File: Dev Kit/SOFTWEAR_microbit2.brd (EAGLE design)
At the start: 61.1 x 28 mm, 16 parts, among them J1 EDGE-80PTH-RA, J2 M22PTH, J3 QWIIC_RIGHT_ANGLE, X1 SM03B-SRSS-TB, X2 SM03B-SRSS-TB, X3 SM03B-SRSS-TB

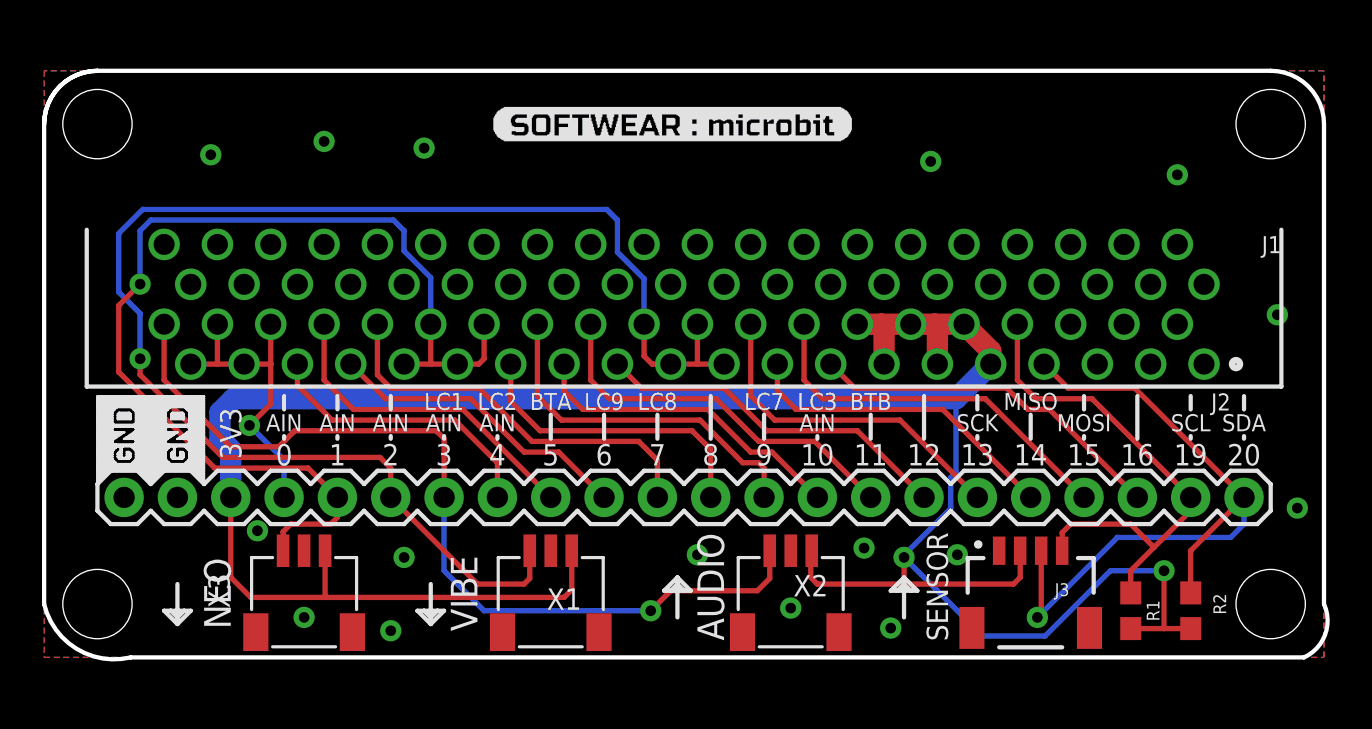
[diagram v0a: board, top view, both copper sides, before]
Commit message: updated design
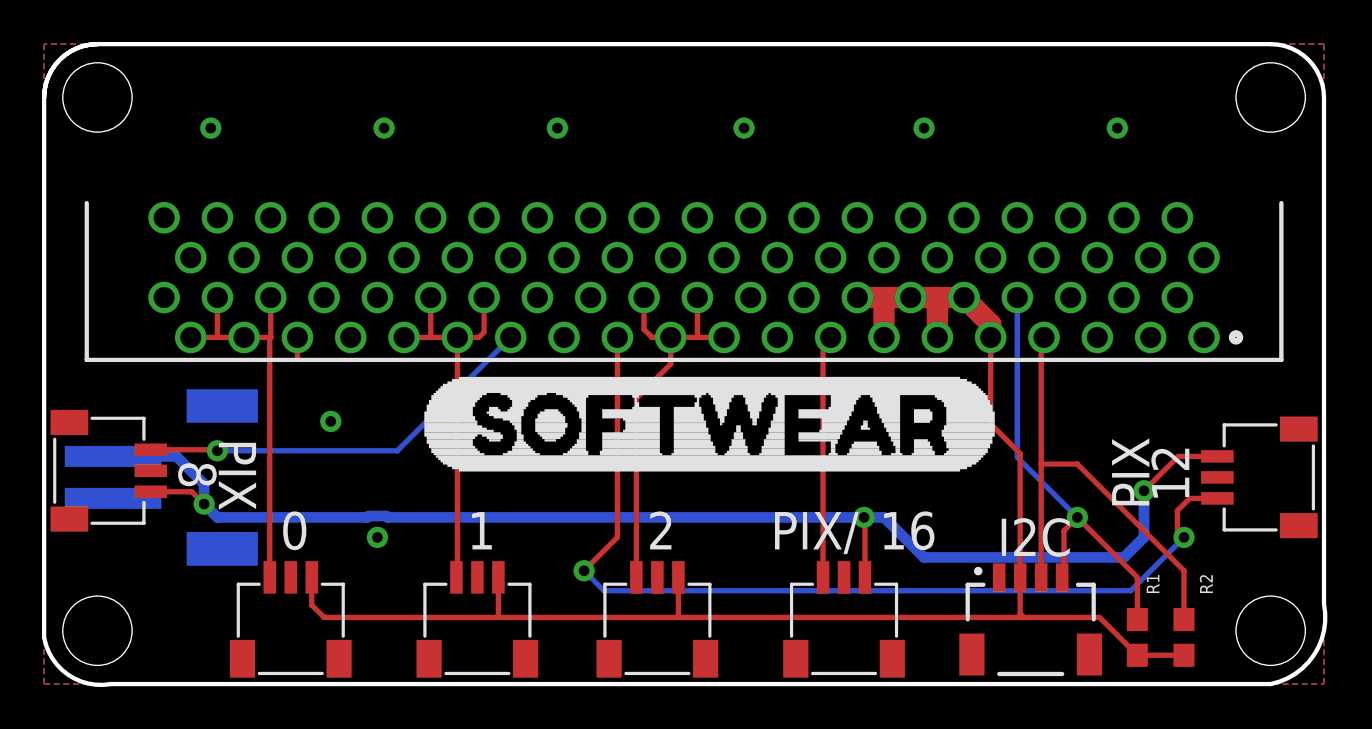
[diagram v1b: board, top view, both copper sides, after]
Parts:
- removed U$2: (no value), negasilk:NEGASILK_MICRO_BIT_BREAKOUT
- removed U$3: (no value), buzzard_labels (21):SOFTWEAR_#_MICROBIT5
- added X4, X5, X6: SM03B-SRSS-TB, con-JST SH (1):SM03B-SRSS-TB
- J2: value M22PTH -> (none); device local_lib:1X22 -> SparkFun-Connectors:JST-2-SMD
- U$1: device negasilk:NEGASILK_MICRO_BIT_BREAKOUT -> buzzard_labels (24):SOFTWEAR0
- moved X2 23.8 mm to (15.6, 5.08)
- moved X3 16.9 mm to (33.0, 5.08)
- moved U$1 15.5 mm to (21.6, 12.4)
- moved X1 3.72 mm to (24.4, 5.08)
- moved J2 3.31 mm to (10.8, 9.84), flipped to the bottom, turned to 90 degrees
- moved R1 1.31 mm to (55.9, 2.22)
- moved R2 1.31 mm to (58.1, 2.22)
- moved J1 1.27 mm to (34.3, 16.5)
- moved H3 1.27 mm to (62.2, 2.54)
- moved H4 1.27 mm to (6.35, 2.54)
- moved H1 1.27 mm to (6.35, 27.9)
- moved H2 1.27 mm to (62.2, 27.9)
- moved J3 1.27 mm to (50.8, 5.08)
- moved FRAME2 0.64 mm to (3.81, -1.27)
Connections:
- removed net 12: J1.A23, J2.16
- removed net 16: J1.A15, J2.20
- removed net 8: J1.A27, J2.12
- removed net AUD: J1.A40, J2.7, X2.1
- removed net NEO: J1.A28, J1.A29, J1.A30, J1.A31, J2.5, X3.1
- removed net VIBE: J1.A19, J1.A20, J1.A21, J1.A22, J2.6, X1.1
- new net 1: J1.A28, J1.A29, J1.A30, J1.A31, X1.1
- new net 2: J1.A19, J1.A20, J1.A21, J1.A22, X3.1
- new net 3: J1.A40
- new net NEO1: J1.A27, X4.1
- new net NEO2: J1.A23, X5.1
- new net NEO3: J1.A15, X6.1
- new net V_BATT: J2.2, X4.3, X5.3, X6.3
- net 0: now also X2.1; no longer J2.4
- net 10: no longer J2.14
- net 11: no longer J2.15
- net 13: no longer J2.17
- net 14: no longer J2.18
- net 15: no longer J2.19
- net 3.3V: no longer J2.3
- net 4: no longer J2.8
- net 5: no longer J2.9
- net 6: no longer J2.10
- net 7: no longer J2.11
- net 9: no longer J2.13
- net GND: now also X4.2, X5.2, X6.2; no longer J2.2
- net SCL: no longer J2.21
- net SDA: no longer J2.22
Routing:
- net VIBE: track 69.4 -> 0.00 mm, vias 1 -> 0
- net V_BATT: track 0.00 -> 64.2 mm, vias 0 -> 3
- net NEO: track 50.2 -> 0.00 mm, vias 1 -> 0
- net 3.3V: track 121.5 -> 73.2 mm, vias 2 -> 0
- net NEO2: track 0.00 -> 45.3 mm, vias 0 -> 2
- net AUD: track 42.3 -> 0.00 mm, vias 1 -> 0
- net 2: track 0.00 -> 19.5 mm
- net NEO1: track 0.00 -> 19.4 mm, vias 0 -> 1
- net 7: track 19.2 -> 0.00 mm
- net 1: track 0.00 -> 18.9 mm
- net 15: track 18.3 -> 0.00 mm
- net 11: track 18.3 -> 0.00 mm
- net 12: track 17.2 -> 0.00 mm
- net 16: track 17.2 -> 0.00 mm
- net 9: track 17.0 -> 0.00 mm
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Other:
- board size 61.1 x 28 mm -> 61 x 30.5 mm
- board text added: "I2C"
- board text added: "PIX"
- board text added: "PIX/"
- board text removed: "10"
- board text removed: "11"
- board text removed: "13"
- board text removed: "14"
- board text removed: "15"
- board text removed: "19"
- board text removed: "20"
- board text removed: "3"
- board text removed: "3V3"
- board text removed: "4"
- board text removed: "5"
- board text removed: "6"
- board text removed: "7"
- board text removed: "9"
- board text removed: "AIN"
- board text removed: "AUDIO"
- board text removed: "BTA"
- board text removed: "BTB"
- board text removed: "LC1"
- board text removed: "LC2"
- board text removed: "LC3"
- board text removed: "LC7"
- board text removed: "LC8"
- board text removed: "LC9"
- board text removed: "MISO"
- board text removed: "MOSI"
- board text removed: "NEO"
- board text removed: "SCK"
- board text removed: "SCL"
- board text removed: "SDA"
- board text removed: "SENSOR"
- board text removed: "VIBE"
